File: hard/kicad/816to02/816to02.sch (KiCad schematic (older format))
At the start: 4 parts, among them U1 65C02 SOCKET, U2 65C816, U3 74HC245, U4 74HC00

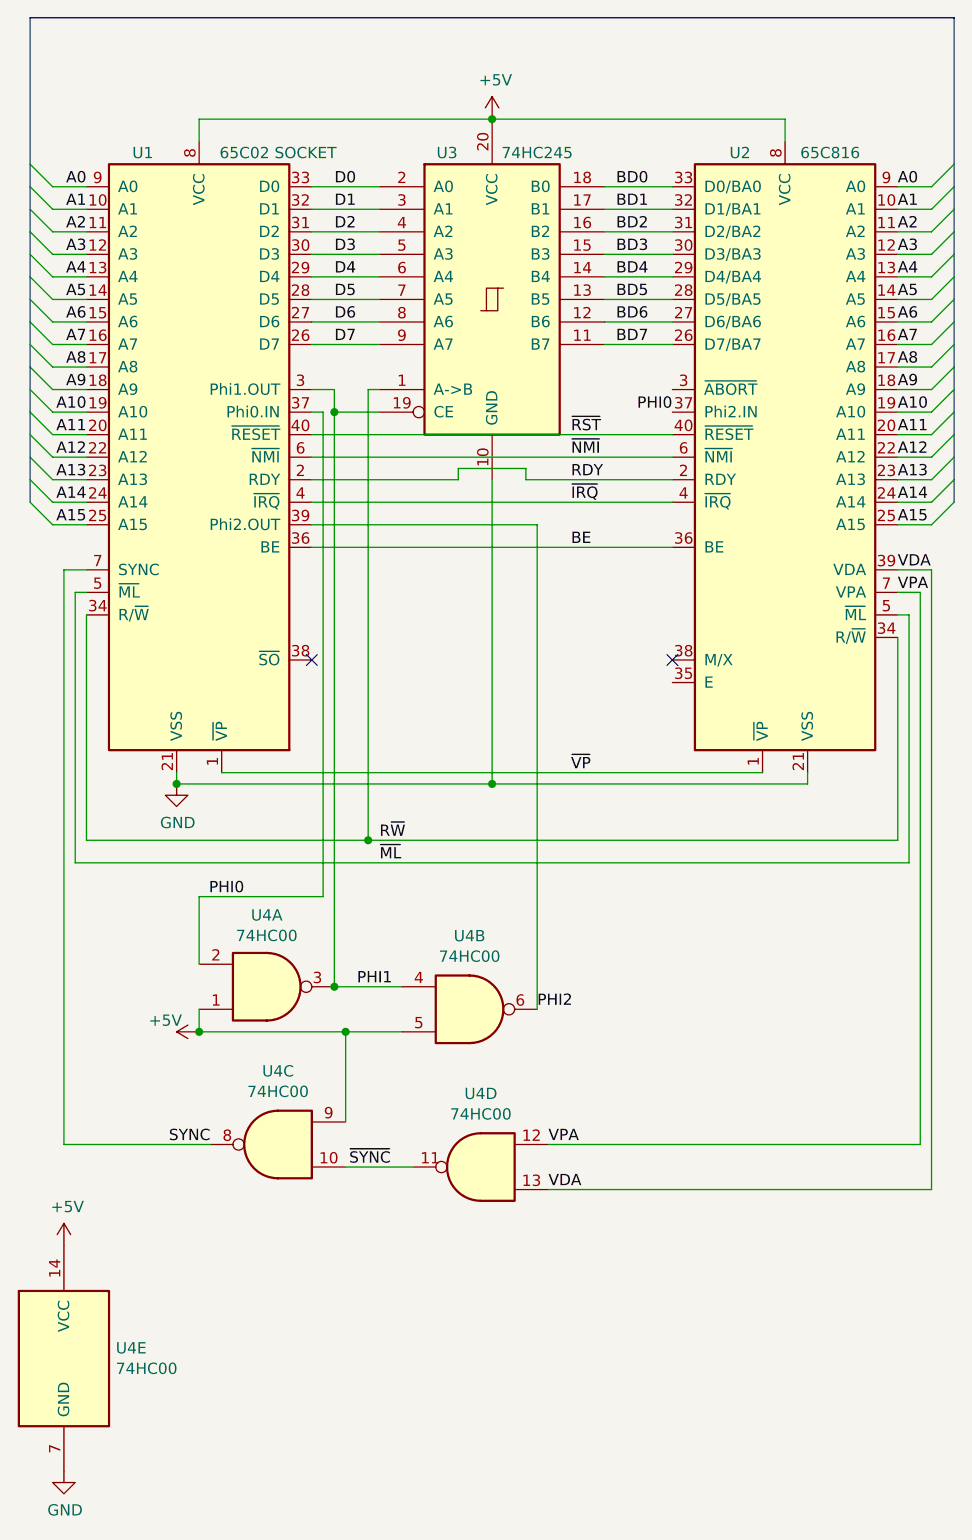
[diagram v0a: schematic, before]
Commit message: updates in adapter
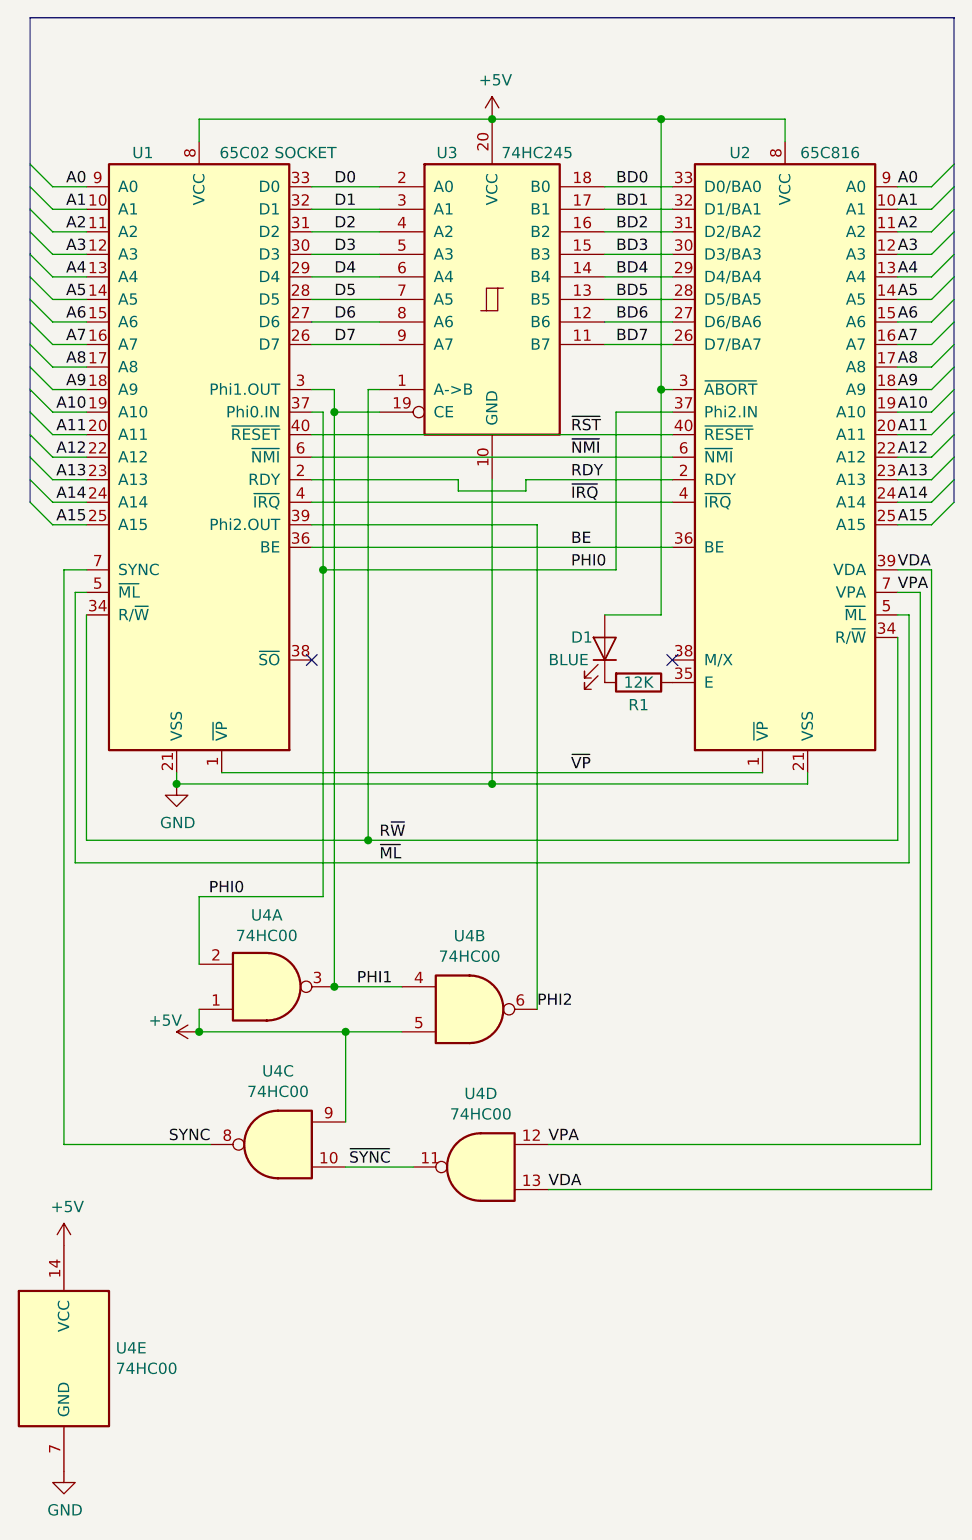
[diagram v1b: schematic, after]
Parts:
- added D1: BLUE, LED_THT:LED_D3.0mm_Horizontal_O6.35mm_Z2.0mm, symbol Device:LED
- added R1: 12K, Resistor_SMD:R_0805_2012Metric_Pad1.15x1.40mm_HandSolder, symbol Device:R
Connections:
- net +5V: now also U2.3 (~ABORT), D1.2 (A)
- net at U2.35 (E): now also R1.1
- new net: D1.1 (K), R1.2
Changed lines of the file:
@@
 EESchema Schematic File Version 4
+LIBS:816to02-cache
 EELAYER 29 0
 EELAYER END
@@
 R~W
 NoConn ~ 3650 3450
-Text Label 3650 2350 2    50   ~ 0
+Text Label 3200 3050 0    50   ~ 0
 PHI0
 Wire Wire Line
@@
 	2050 2650 2700 2650
 Wire Wire Line
-	2700 2650 2700 2600
-Wire Wire Line
-	2700 2600 3000 2600
-Wire Wire Line
-	3000 2600 3000 2650
+	2700 2650 2700 2700
+Wire Wire Line
+	3000 2700 3000 2650
 Wire Wire Line
 	3000 2650 3650 2650
@@
 	2050 2350 2100 2350
 Wire Wire Line
-	2100 2350 2100 4500
+	2100 2350 2100 3050
 Wire Wire Line
 	2100 4500 1550 4500
@@
 Connection ~ 2850 1050
 Wire Wire Line
-	2850 1050 4150 1050
+	2850 1050 3600 1050
 $Comp
 L power:+5V #PWR0103
@@
 	1    0    0    -1
 $EndComp
+Wire Wire Line
+	2700 2700 3000 2700
+Wire Wire Line
+	2100 3050 3400 3050
+Wire Wire Line
+	3400 3050 3400 2350
+Wire Wire Line
+	3400 2350 3650 2350
+Connection ~ 2100 3050
+Wire Wire Line
+	2100 3050 2100 4500
+Wire Wire Line
+	3650 2250 3600 2250
+Wire Wire Line
+	3600 2250 3600 1050
+Connection ~ 3600 1050
+Wire Wire Line
+	3600 1050 4150 1050
+$Comp
+L Device:R R1
+U 1 1 649BA6B6
+P 3500 3550
+F 0 "R1" V 3600 3550 50  0000 C CNN
+F 1 "12K" V 3500 3550 50  0000 C CNN
+F 2 "Resistor_SMD:R_0805_2012Metric_Pad1.15x1.40mm_HandSolder" V 3430 3550 50  0001 C CNN
+F 3 "~" H 3500 3550 50  0001 C CNN
+	1    3500 3550
+	0    1    1    0
+$EndComp
+$Comp
+L Device:LED D1
+U 1 1 649BBBF1
+P 3350 3400
+F 0 "D1" V 3400 3250 50  0000 L CNN
+F 1 "BLUE" V 3300 3150 50  0000 L CNN
+F 2 "LED_THT:LED_D3.0mm_Horizontal_O6.35mm_Z2.0mm" H 3350 3400 50  0001 C CNN
+F 3 "~" H 3350 3400 50  0001 C CNN
+	1    3350 3400
+	0    1    -1   0
+$EndComp
+Wire Wire Line
+	3350 3250 3600 3250
+Wire Wire Line
+	3600 3250 3600 2250
 Wire Bus Line
 	4900 600  4900 2750
 Wire Bus Line
 	800  600  800  2750
+Connection ~ 3600 2250
 $EndSCHEMATC
